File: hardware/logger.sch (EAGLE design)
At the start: 40 parts, among them J1 MICRO_USB_B_HIROSE_ZX62-B-5PA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, SW1 TVAF06-A020B-R, U1 RX-8035LC, U2 NJM12888F, X1 FA-238

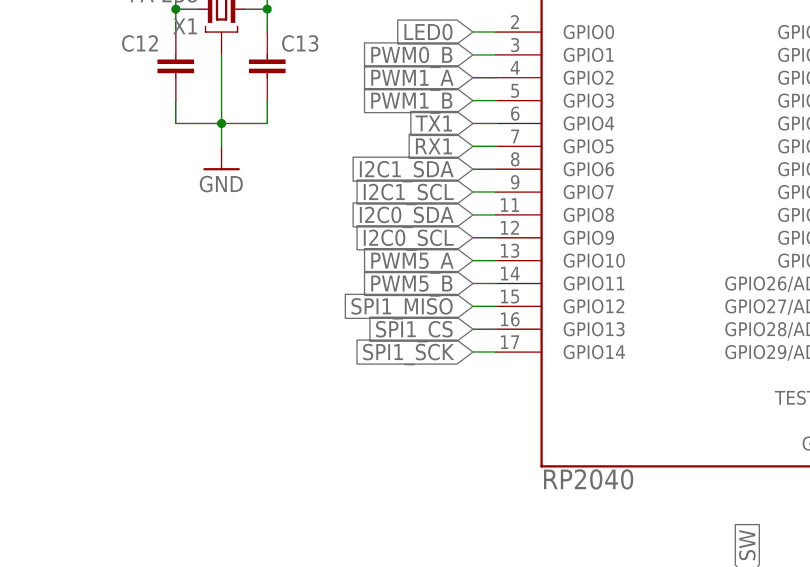
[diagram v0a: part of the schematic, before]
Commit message: 若干修正
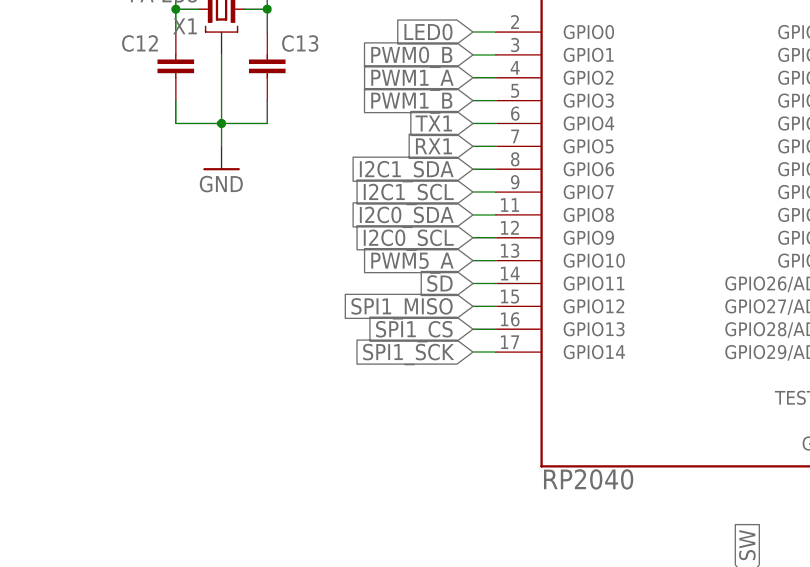
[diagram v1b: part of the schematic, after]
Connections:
- removed net PWM5_B: RP1.GPIO11
- net SD: now also RP1.GPIO11
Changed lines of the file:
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@@
-</segment>
-</net>
-<net name="PWM5_B" class="0">
-<segment>
-<pinref part="RP1" gate="G$1" pin="GPIO11"/>
-<wire x1="33.02" y1="68.58" x2="30.48" y2="68.58" width="0.1524" layer="91"/>
-<label x="30.48" y="68.58" size="1.778" layer="95" rot="R180" xref="yes"/>
 </segment>
 </net>
@@
 <label x="213.36" y="63.5" size="1.778" layer="95" rot="R180" xref="yes"/>
 </segment>
+<segment>
+<pinref part="RP1" gate="G$1" pin="GPIO11"/>
+<wire x1="33.02" y1="68.58" x2="30.48" y2="68.58" width="0.1524" layer="91"/>
+<label x="30.48" y="68.58" size="1.778" layer="95" rot="R180" xref="yes"/>
+</segment>
 </net>
